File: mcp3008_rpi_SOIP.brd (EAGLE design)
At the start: 44.8 x 20.3 mm, 4 parts

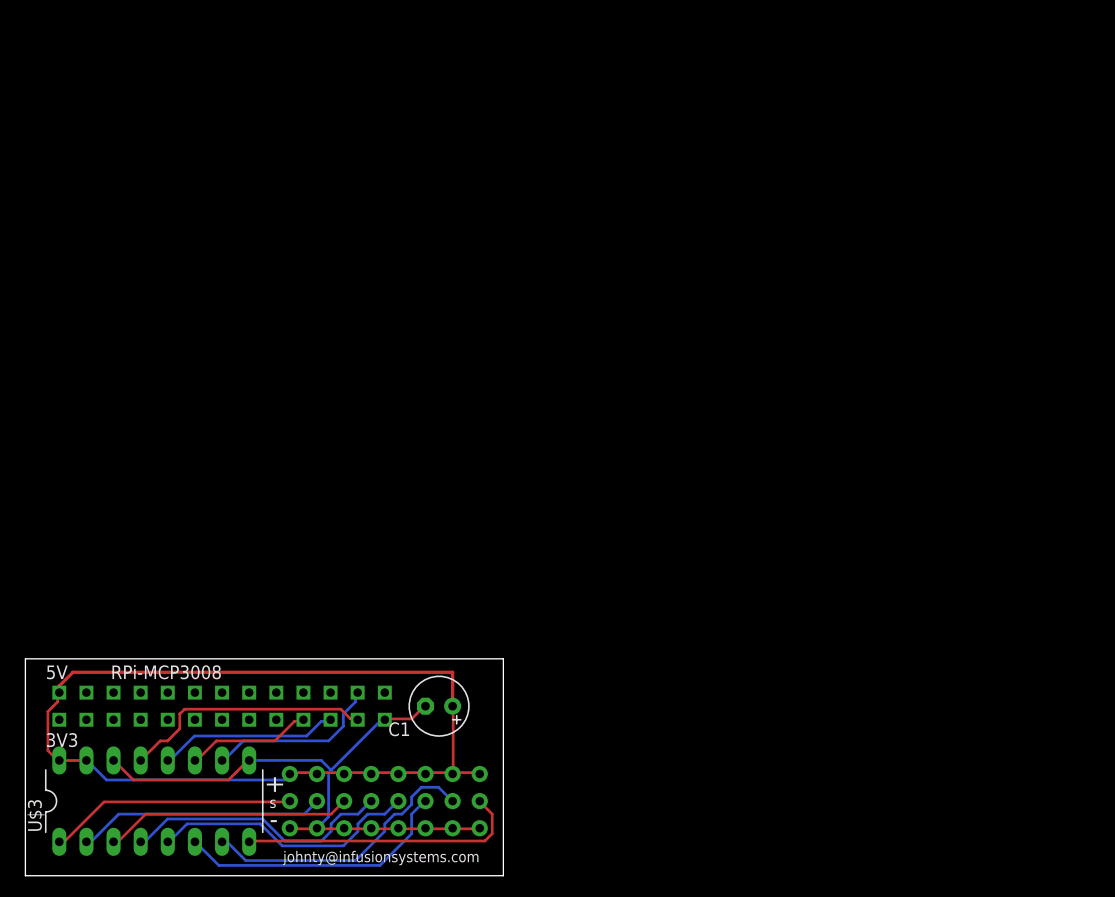
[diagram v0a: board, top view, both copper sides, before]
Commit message: i2c board complete
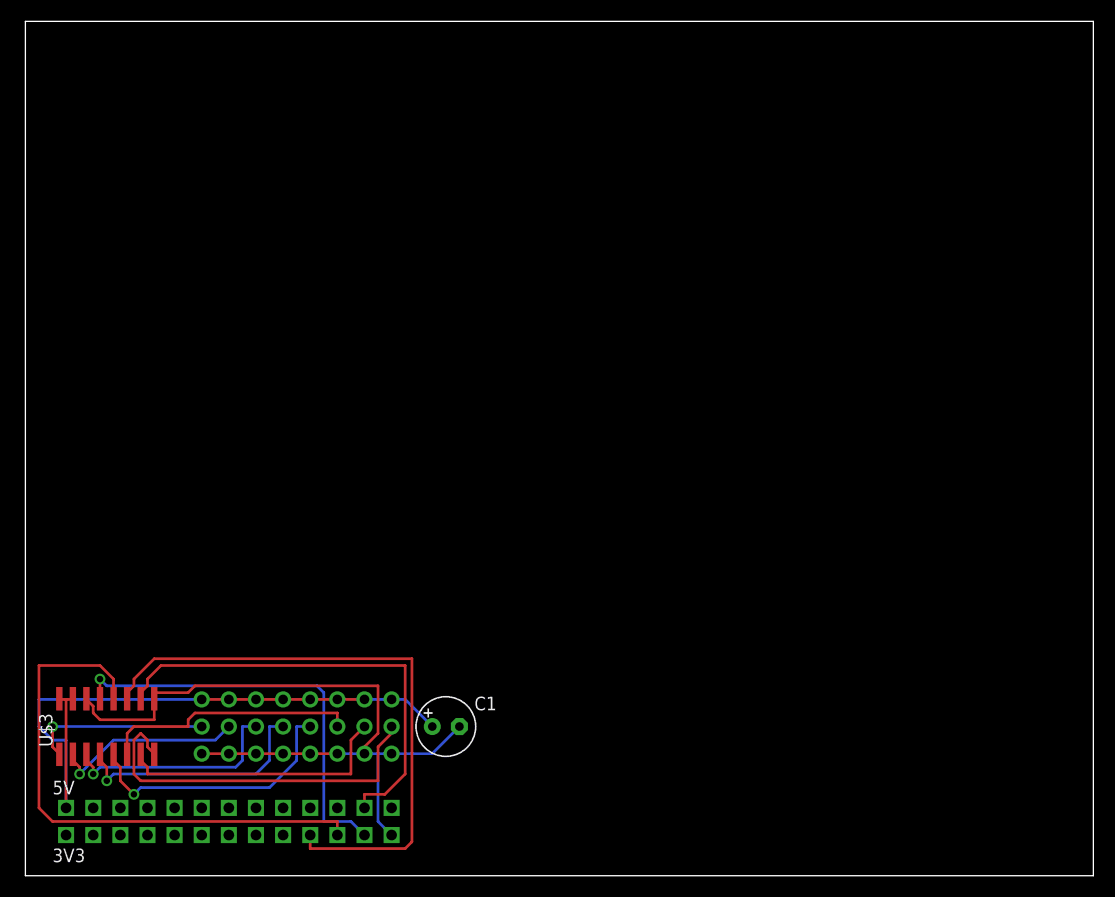
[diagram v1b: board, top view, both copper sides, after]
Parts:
- U$1: value 3BY8 -> 3BY83X8_SAMTEC
- U$3: value MCP3008P -> MCP3008SL; device MCP3008:DIL16 -> MCP3008:SO16
- moved U$2 10.8 mm to (17.8, 5.08)
- moved U$1 10.8 mm to (21.6, 15.2)
- moved U$3 8.28 mm to (7.62, 14.0)
- moved C1 2.01 mm to (39.4, 14.0), turned to 0 degrees
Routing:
- net N$11: track 11.7 -> 57.1 mm
- net N$9: track 16.8 -> 52.4 mm
- net VCC: track 95.9 -> 61.4 mm
- net N$12: track 16.4 -> 42.8 mm
- net N$10: track 23.5 -> 39.7 mm, vias 0 -> 1
- net GND: track 57.6 -> 71.5 mm
- net N$8: track 26.6 -> 35.3 mm
- net N$1: track 23.2 -> 16.8 mm, vias 0 -> 1
- net N$2: track 23.2 -> 17.9 mm, vias 0 -> 1
- net N$3: track 23.2 -> 21.0 mm, vias 0 -> 1
- net N$4: track 25.3 -> 23.2 mm, vias 0 -> 1
- net N$6: track 26.0 -> 24.1 mm
- net N$5: track 25.2 -> 25.5 mm, vias 0 -> 1
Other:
- board size 44.8 x 20.3 mm -> 100 x 80 mm
- board text removed: "+"
- board text removed: "-"
- board text removed: "RPi-MCP3008"
- board text removed: "johnty@infusionsystems.com"
- board text removed: "s"
